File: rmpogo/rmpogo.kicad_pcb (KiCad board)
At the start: 2 copper layers, 11.9 x 63.5 mm, 2 parts, among them J1 USB_B_Micro, J2 Conn_01x05_Male

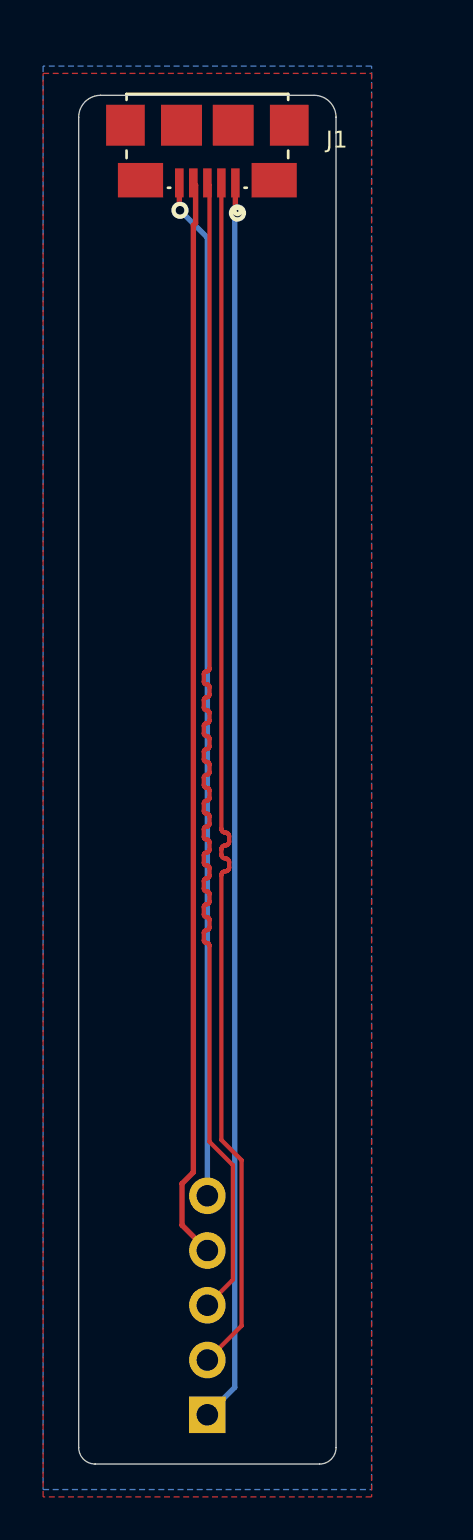
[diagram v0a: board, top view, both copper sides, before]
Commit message: this is better, me thinks
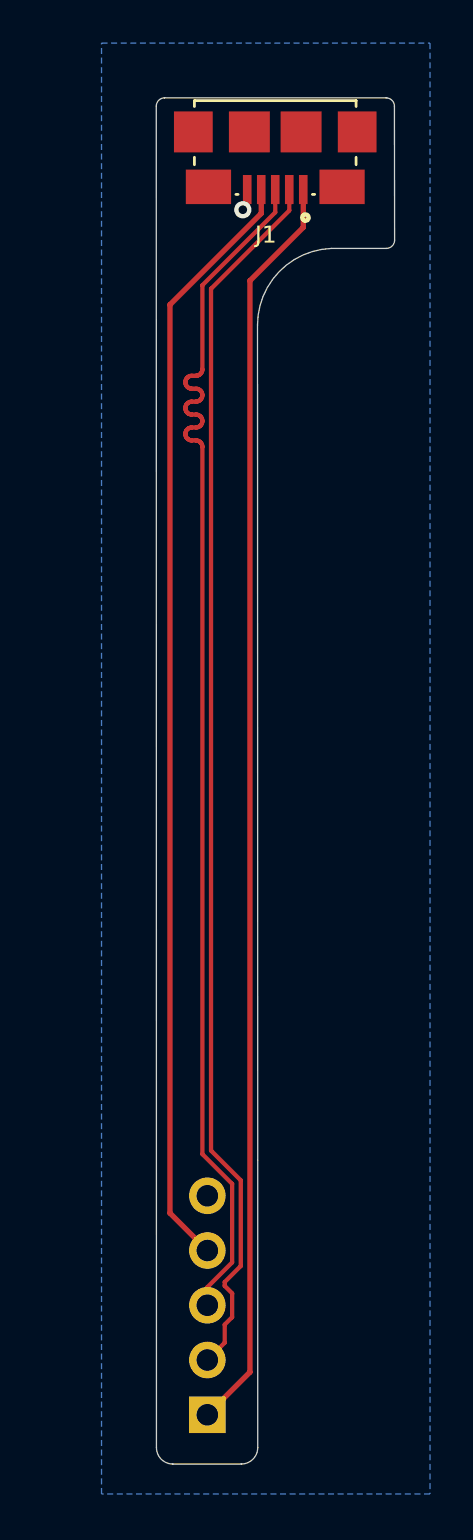
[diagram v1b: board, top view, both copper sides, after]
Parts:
- moved J1 3.17 mm to (138.2, 60.2)
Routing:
- net /GND: track 47.5 -> 1.02 mm
- net Net-(J1-Pad4): track 50.3 -> 51.7 mm
- net /D+: track 56.4 -> 57.4 mm
- net /VBUS: track 57.8 -> 58.7 mm, vias 1 -> 0
- net /D-: track 56.5 -> 57.3 mm
- removed copper zone on F.Cu, net /VBUS
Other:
- board size 11.9 x 63.5 mm -> 11.1 x 63.4 mm
